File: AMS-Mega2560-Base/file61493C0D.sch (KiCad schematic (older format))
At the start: 29 parts, among them IC1 LM2670SX-5.0_NOPB, IC18 TL071CP, IC2 LM2597MX-ADJ_NOPB, J1 Screw_Terminal_01x02, Q1 IRF9Z34NPBF, U1 BK_HTC-15M

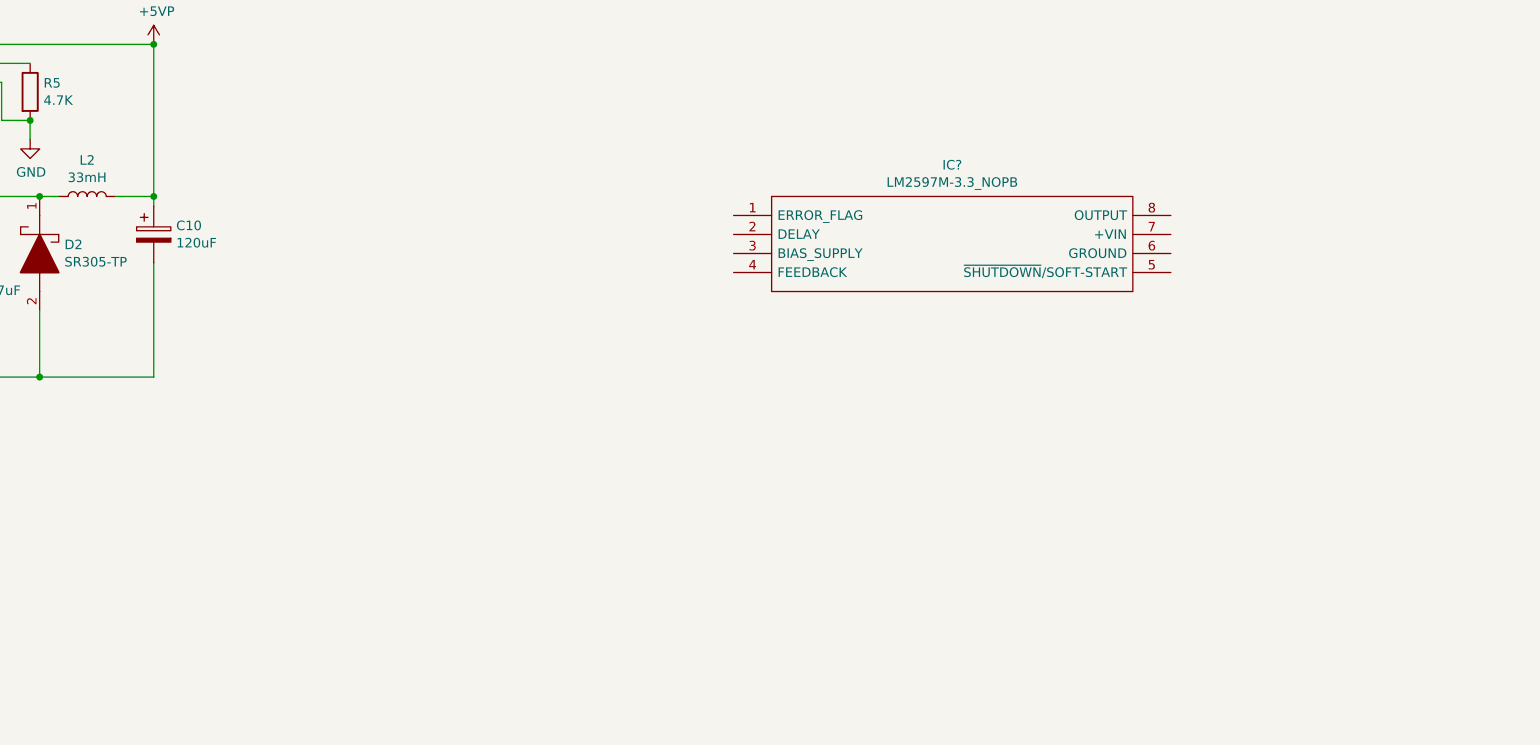
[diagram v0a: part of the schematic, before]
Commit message: wip working on it.
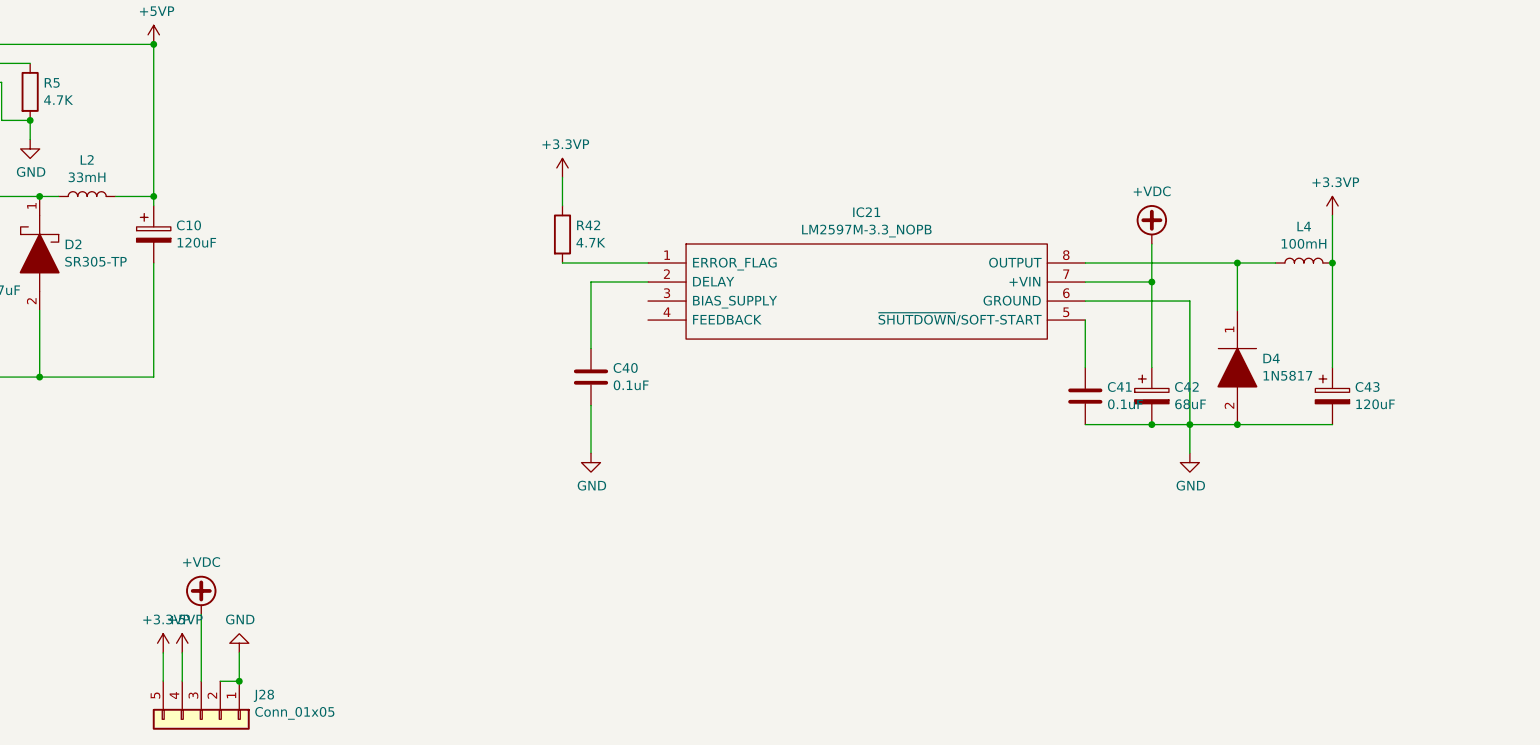
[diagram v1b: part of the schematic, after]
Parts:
- added C40, C41: 0.1uF, Capacitor_THT:C_Rect_L9.0mm_W3.6mm_P7.50mm_MKT, symbol Device:C
- added C42: 68uF, Capacitor_THT:CP_Radial_D5.0mm_P2.50mm, symbol Device:CP
- added C43: 120uF, Capacitor_THT:CP_Radial_D8.0mm_P5.00mm, symbol Device:CP
- added D4: 1N5817, SamacSys_Parts:DIOAD1414W86L464D238, symbol SamacSys_Parts:1N5817
- added J28: Conn_01x05, symbol Connector_Generic:Conn_01x05
- added L4: 100mH, Inductor_THT:L_Axial_L9.5mm_D4.0mm_P15.24mm_Horizontal_Fastron_SMCC, symbol Device:L
- added R42: 4.7K, Resistor_THT:R_Axial_DIN0207_L6.3mm_D2.5mm_P2.54mm_Vertical, symbol Device:R
- gave numbers to parts that had none: 1
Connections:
- net +5VP: now also J28.4 (Pin_4)
- net +VDC: now also IC21.7 (+VIN), C42.1, J28.3 (Pin_3)
- net GND: now also IC21.6 (GROUND), C40.2, C41.2, C42.2, C43.2, D4.2, J28.1 (Pin_1), J28.2 (Pin_2)
- net at IC21.1 (ERROR_FLAG): now also R42.2
- net at IC21.2 (DELAY): now also C40.1
- net at IC21.5 (~SHUTDOWN~/SOFT-START): now also C41.1
- net at IC21.8 (OUTPUT): now also D4.1, L4.1
- new net +3.3VP: C43.1, J28.5 (Pin_5), L4.2, R42.1
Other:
- moved on the sheet: IC21
